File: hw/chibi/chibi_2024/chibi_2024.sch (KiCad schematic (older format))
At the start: 85 parts, among them P1 VIN, P3 GND, P4 CONN_02X05, P5 SWD, Q1 AO3415A, Q10 Q_NPN_CBE, Q11 Q_NPN_CBE, Q2 AO3415A, Q3 AO3415A, Q4 AO3415A, Q5 AO3415A, Q6 AO3415A, Q7 AO3415A, Q8 AO3415A, Q9 Q_PNP_CBE, SW1 USER, SW2 RESET, U1 LD1117S33CTR, U2 SP3485CN, U3 STM32F030F4Px, U4 LM358, U5 74HC595_mine, U6 LM393, U7 74HC595_mine, Y1 8MHz

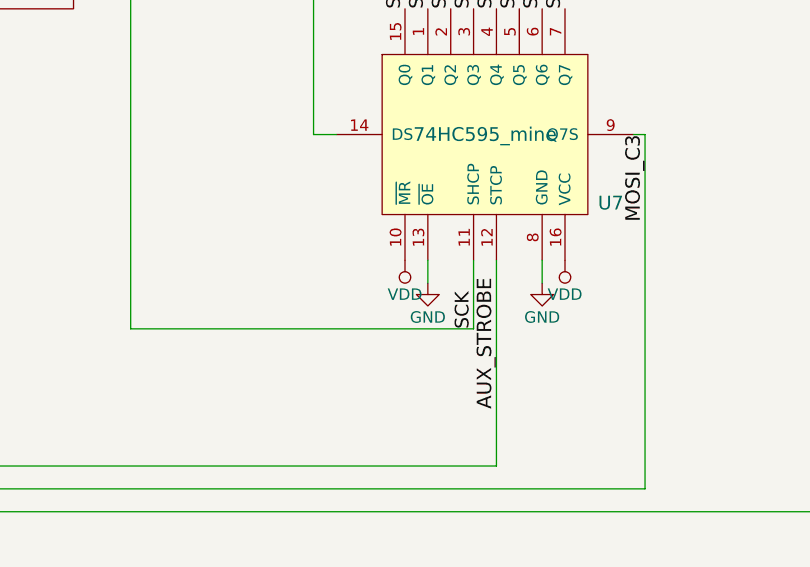
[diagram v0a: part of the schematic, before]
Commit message: Layout mostly done
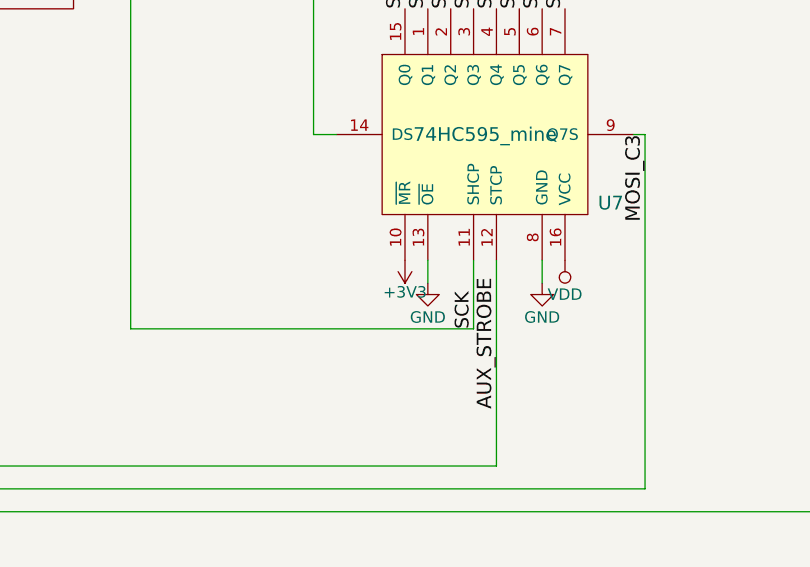
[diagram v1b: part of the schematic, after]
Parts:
- C19, C3: footprint Capacitors_ThroughHole:C_Radial_D10_L20_P5-7.5 -> Capacitors_ThroughHole:C_Radial_D10_L20_P5
- D1: footprint Discret:D5 -> Discret:D3
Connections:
- net +3V3: now also U7.10 (~MR)
- net VDD: no longer U7.10 (~MR)
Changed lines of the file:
@@
 F 0 "C3" H 15200 4150 50  0000 L CNN
 F 1 "1000u" H 15150 3900 50  0000 L CNN
-F 2 "Capacitors_ThroughHole:C_Radial_D10_L20_P5-7.5" H 15438 3850 50  0001 C CNN
+F 2 "Capacitors_ThroughHole:C_Radial_D10_L20_P5" H 15438 3850 50  0001 C CNN
 F 3 "" H 15400 4000 50  0000 C CNN
 F 4 "RAD FR 1.000/25" H 15400 3750 60  0000 C CNN "Reichelt"
@@
 	1    13000 12700
 	-1   0    0    -1
-$EndComp
-$Comp
-L VDD #PWR018
-U 1 1 5903D437
-P 12900 12600
-F 0 "#PWR018" H 12900 12450 50  0001 C CNN
-F 1 "VDD" H 12900 12750 50  0000 C CNN
-F 2 "" H 12900 12600 50  0000 C CNN
-F 3 "" H 12900 12600 50  0000 C CNN
-	1    12900 12600
-	1    0    0    1
 $EndComp
 $Comp
@@
 F 0 "C19" H 14750 10150 50  0000 L CNN
 F 1 "1000u" H 14700 9900 50  0000 L CNN
-F 2 "Capacitors_ThroughHole:C_Radial_D10_L20_P5-7.5" H 14988 9850 50  0001 C CNN
+F 2 "Capacitors_ThroughHole:C_Radial_D10_L20_P5" H 14988 9850 50  0001 C CNN
 F 3 "" H 14950 10000 50  0000 C CNN
 	1    14950 10000
@@
 F 0 "D1" H 14800 4100 50  0000 C CNN
 F 1 "6.4V 1.3W" V 15000 4000 50  0000 C CNN
-F 2 "Discret:D5" H 14800 4000 50  0001 C CNN
+F 2 "Discret:D3" H 14800 4000 50  0001 C CNN
 F 3 "" H 14800 4000 50  0000 C CNN
 	1    14800 4000
@@
 Wire Wire Line
 	5850 12000 4600 12000
+$Comp
+L +3V3 #PWR?
+U 1 1 590A17BD
+P 12900 12600
+F 0 "#PWR?" H 12900 12450 50  0001 C CNN
+F 1 "+3V3" H 12900 12740 50  0000 C CNN
+F 2 "" H 12900 12600 50  0000 C CNN
+F 3 "" H 12900 12600 50  0000 C CNN
+	1    12900 12600
+	-1   0    0    1
+$EndComp
 $EndSCHEMATC

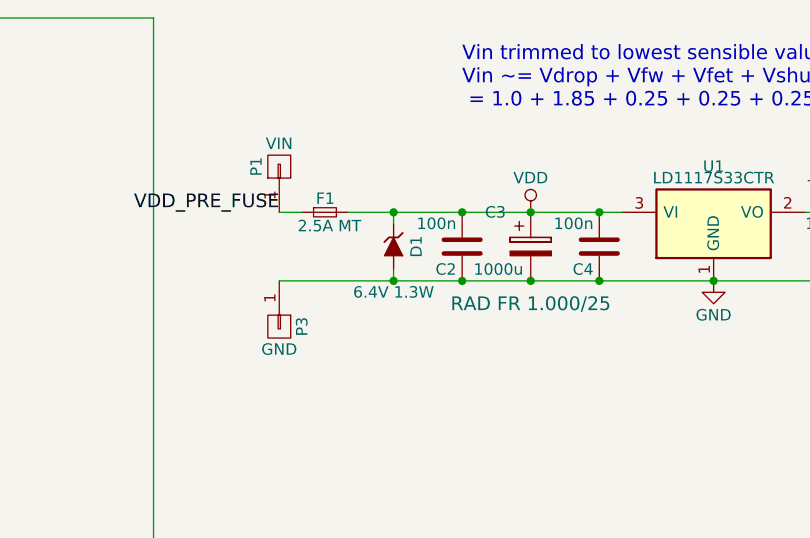
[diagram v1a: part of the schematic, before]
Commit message: Design mostly done
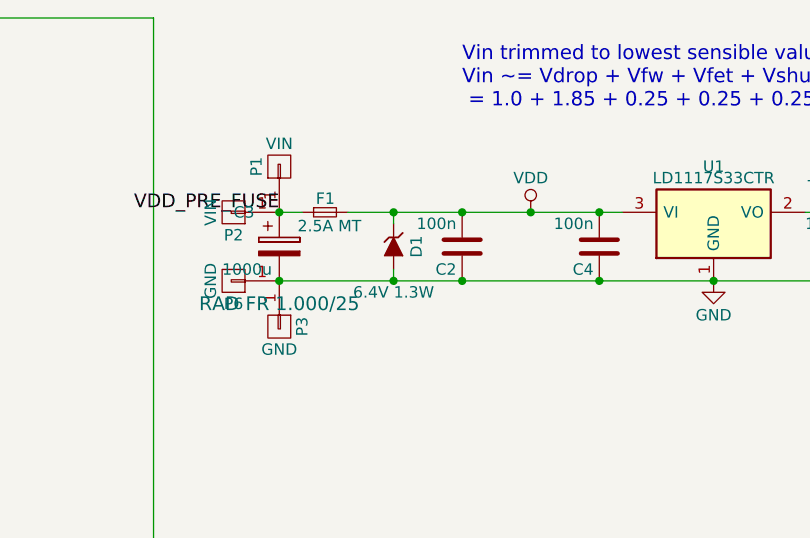
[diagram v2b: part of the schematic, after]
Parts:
- added P2: VIN, footprints:spade_6.35mm, symbol CONN_01X01
- added P6: GND, footprints:spade_6.35mm, symbol CONN_01X01
- SW1, SW2: footprint Buttons_Switches_ThroughHole:SW_PUSH_SMALL -> Buttons_Switches_SMD:SW_SPST_FSMSM
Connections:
- net GND: now also P6.1 (P1)
- net VDD: no longer C3.1
- net VDD_PRE_FUSE: now also C3.1, P2.1 (P1)
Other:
- moved on the sheet: C3
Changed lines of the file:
@@
 L CP C3
 U 1 1 5901F62F
-P 15400 4000
-F 0 "C3" H 15200 4150 50  0000 L CNN
-F 1 "1000u" H 15150 3900 50  0000 L CNN
-F 2 "Capacitors_ThroughHole:C_Radial_D10_L20_P5" H 15438 3850 50  0001 C CNN
-F 3 "" H 15400 4000 50  0000 C CNN
-F 4 "RAD FR 1.000/25" H 15400 3750 60  0000 C CNN "Reichelt"
-	1    15400 4000
+P 14300 4000
+F 0 "C3" H 14100 4150 50  0000 L CNN
+F 1 "1000u" H 14050 3900 50  0000 L CNN
+F 2 "Capacitors_ThroughHole:C_Radial_D10_L20_P5" H 14338 3850 50  0001 C CNN
+F 3 "" H 14300 4000 50  0000 C CNN
+F 4 "RAD FR 1.000/25" H 14300 3750 60  0000 C CNN "Reichelt"
+	1    14300 4000
 	1    0    0    -1
 $EndComp
@@
 $EndComp
 $Comp
-L GND #PWR019
+L GND #PWR018
 U 1 1 5905739D
 P 4850 13300
-F 0 "#PWR019" H 4850 13050 50  0001 C CNN
+F 0 "#PWR018" H 4850 13050 50  0001 C CNN
 F 1 "GND" H 4850 13150 50  0000 C CNN
 F 2 "" H 4850 13300 50  0000 C CNN
@@
 $EndComp
 $Comp
-L +3V3 #PWR020
+L +3V3 #PWR019
 U 1 1 59059547
 P 2750 3850
-F 0 "#PWR020" H 2750 3700 50  0001 C CNN
+F 0 "#PWR019" H 2750 3700 50  0001 C CNN
 F 1 "+3V3" H 2750 3990 50  0000 C CNN
 F 2 "" H 2750 3850 50  0000 C CNN
@@
 $EndComp
 $Comp
-L GND #PWR021
+L GND #PWR020
 U 1 1 5905B96D
 P 7150 6800
-F 0 "#PWR021" H 7150 6550 50  0001 C CNN
+F 0 "#PWR020" H 7150 6550 50  0001 C CNN
 F 1 "GND" H 7150 6650 50  0000 C CNN
 F 2 "" H 7150 6800 50  0000 C CNN
@@
 $EndComp
 $Comp
-L +3V3 #PWR022
+L +3V3 #PWR021
 U 1 1 5905BCF8
 P 7050 6300
-F 0 "#PWR022" H 7050 6150 50  0001 C CNN
+F 0 "#PWR021" H 7050 6150 50  0001 C CNN
 F 1 "+3V3" H 7050 6440 50  0000 C CNN
 F 2 "" H 7050 6300 50  0000 C CNN
@@
 $EndComp
 $Comp
-L VDD #PWR023
+L VDD #PWR022
 U 1 1 5905CD8E
 P 15400 3850
-F 0 "#PWR023" H 15400 3700 50  0001 C CNN
+F 0 "#PWR022" H 15400 3700 50  0001 C CNN
 F 1 "VDD" H 15400 4000 50  0000 C CNN
 F 2 "" H 15400 3850 50  0000 C CNN
@@
 F 0 "SW1" H 7730 3810 50  0000 C CNN
 F 1 "USER" H 7650 3650 50  0000 C CNN
-F 2 "Buttons_Switches_ThroughHole:SW_PUSH_SMALL" H 7650 3900 50  0001 C CNN
+F 2 "Buttons_Switches_SMD:SW_SPST_FSMSM" H 7650 3900 50  0001 C CNN
 F 3 "" H 7650 3900 50  0000 C CNN
 	1    7650 3700
@@
 F 0 "SW2" H 3080 4810 50  0000 C CNN
 F 1 "RESET" H 3000 4650 50  0000 C CNN
-F 2 "Buttons_Switches_ThroughHole:SW_PUSH_SMALL" H 3000 4900 50  0001 C CNN
+F 2 "Buttons_Switches_SMD:SW_SPST_FSMSM" H 3000 4900 50  0001 C CNN
 F 3 "" H 3000 4900 50  0000 C CNN
 	1    3000 4700
@@
 $EndComp
 $Comp
-L GND #PWR024
+L GND #PWR023
 U 1 1 59065530
 P 14950 10250
-F 0 "#PWR024" H 14950 10000 50  0001 C CNN
+F 0 "#PWR023" H 14950 10000 50  0001 C CNN
 F 1 "GND" H 14950 10100 50  0000 C CNN
 F 2 "" H 14950 10250 50  0000 C CNN
@@
 CM_STAGE2_FB
 $Comp
-L VDD #PWR025
+L VDD #PWR024
 U 1 1 5906AB80
 P 16200 6800
-F 0 "#PWR025" H 16200 6650 50  0001 C CNN
+F 0 "#PWR024" H 16200 6650 50  0001 C CNN
 F 1 "VDD" H 16200 6950 50  0000 C CNN
 F 2 "" H 16200 6800 50  0000 C CNN
@@
 $EndComp
 $Comp
-L GND #PWR026
+L GND #PWR025
 U 1 1 5906CB51
 P 15750 6500
-F 0 "#PWR026" H 15750 6250 50  0001 C CNN
+F 0 "#PWR025" H 15750 6250 50  0001 C CNN
 F 1 "GND" H 15750 6350 50  0000 C CNN
 F 2 "" H 15750 6500 50  0000 C CNN
@@
 $EndComp
 $Comp
-L GND #PWR027
+L GND #PWR026
 U 1 1 5906EF8A
 P 16700 6500
-F 0 "#PWR027" H 16700 6250 50  0001 C CNN
+F 0 "#PWR026" H 16700 6250 50  0001 C CNN
 F 1 "GND" H 16700 6350 50  0000 C CNN
 F 2 "" H 16700 6500 50  0000 C CNN
@@
 CMEAS_OFFX_COMP
 $Comp
-L GND #PWR028
+L GND #PWR027
 U 1 1 59071D5D
 P 7750 3950
-F 0 "#PWR028" H 7750 3700 50  0001 C CNN
+F 0 "#PWR027" H 7750 3700 50  0001 C CNN
 F 1 "GND" H 7750 3800 50  0000 C CNN
 F 2 "" H 7750 3950 50  0000 C CNN
@@
 $EndComp
 $Comp
-L +3V3 #PWR029
+L +3V3 #PWR028
 U 1 1 590927CA
 P 16950 7600
-F 0 "#PWR029" H 16950 7450 50  0001 C CNN
+F 0 "#PWR028" H 16950 7450 50  0001 C CNN
 F 1 "+3V3" H 16950 7740 50  0000 C CNN
 F 2 "" H 16950 7600 50  0000 C CNN
@@
 Vin trimmed to lowest sensible value to reduce power dissipation.\nVin ~~= Vdrop + Vfw + Vfet + Vshunt + Vwiring\n = 1.0 + 1.85 + 0.25 + 0.25 + 0.25 = 3.6V
 $Comp
-L +3V3 #PWR030
+L +3V3 #PWR029
 U 1 1 59098A31
 P 8550 5050
-F 0 "#PWR030" H 8550 4900 50  0001 C CNN
+F 0 "#PWR029" H 8550 4900 50  0001 C CNN
 F 1 "+3V3" H 8550 5190 50  0000 C CNN
 F 2 "" H 8550 5050 50  0000 C CNN
@@
 $EndComp
 $Comp
-L +3V3 #PWR031
+L +3V3 #PWR030
 U 1 1 590D225D
 P 6900 9900
-F 0 "#PWR031" H 6900 9750 50  0001 C CNN
+F 0 "#PWR030" H 6900 9750 50  0001 C CNN
 F 1 "+3V3" H 6900 10040 50  0000 C CNN
 F 2 "" H 6900 9900 50  0000 C CNN
@@
 $EndComp
 $Comp
-L GND #PWR032
+L GND #PWR031
 U 1 1 590E4406
 P 7750 13000
-F 0 "#PWR032" H 7750 12750 50  0001 C CNN
+F 0 "#PWR031" H 7750 12750 50  0001 C CNN
 F 1 "GND" H 7750 12850 50  0000 C CNN
 F 2 "" H 7750 13000 50  0000 C CNN
@@
 SCK
 $Comp
-L +3V3 #PWR033
+L +3V3 #PWR032
 U 1 1 590F5DC8
 P 5450 10850
-F 0 "#PWR033" H 5450 10700 50  0001 C CNN
+F 0 "#PWR032" H 5450 10700 50  0001 C CNN
 F 1 "+3V3" V 5350 10900 50  0000 C CNN
 F 2 "" H 5450 10850 50  0000 C CNN
@@
 $EndComp
 $Comp
-L GND #PWR034
+L GND #PWR033
 U 1 1 590F5FC2
 P 5550 10850
-F 0 "#PWR034" H 5550 10600 50  0001 C CNN
+F 0 "#PWR033" H 5550 10600 50  0001 C CNN
 F 1 "GND" H 5550 10700 50  0000 C CNN
 F 2 "" H 5550 10850 50  0000 C CNN
@@
 $EndComp
 $Comp
-L GND #PWR035
+L GND #PWR034
 U 1 1 590F70E3
 P 6050 10850
-F 0 "#PWR035" H 6050 10600 50  0001 C CNN
+F 0 "#PWR034" H 6050 10600 50  0001 C CNN
 F 1 "GND" H 6050 10700 50  0000 C CNN
 F 2 "" H 6050 10850 50  0000 C CNN
@@
 $EndComp
 $Comp
-L +3V3 #PWR036
+L +3V3 #PWR035
 U 1 1 590F8493
 P 6150 10850
-F 0 "#PWR036" H 6150 10700 50  0001 C CNN
+F 0 "#PWR035" H 6150 10700 50  0001 C CNN
 F 1 "+3V3" V 6250 10900 50  0000 C CNN
 F 2 "" H 6150 10850 50  0000 C CNN
@@
 MOSI_C3
 $Comp
-L GND #PWR037
+L GND #PWR036
 U 1 1 590FF5A0
 P 8900 5150
-F 0 "#PWR037" H 8900 4900 50  0001 C CNN
+F 0 "#PWR036" H 8900 4900 50  0001 C CNN
 F 1 "GND" H 8900 5000 50  0000 C CNN
 F 2 "" H 8900 5150 50  0000 C CNN
@@
 Wire Wire Line
 	14300 4150 18150 4150
-Connection ~ 15400 4150
-Connection ~ 15400 3850
 Wire Wire Line
 	16600 3850 18150 3850
@@
 $EndComp
 $Comp
-L +3V3 #PWR038
+L +3V3 #PWR037
 U 1 1 590B5F7D
 P 19300 11150
-F 0 "#PWR038" H 19300 11000 50  0001 C CNN
+F 0 "#PWR037" H 19300 11000 50  0001 C CNN
 F 1 "+3V3" H 19300 11290 50  0000 C CNN
 F 2 "" H 19300 11150 50  0000 C CNN
@@
 $EndComp
 $Comp
-L +3V3 #PWR039
+L +3V3 #PWR038
 U 1 1 590AABFE
 P 18300 10800
-F 0 "#PWR039" H 18300 10650 50  0001 C CNN
+F 0 "#PWR038" H 18300 10650 50  0001 C CNN
 F 1 "+3V3" H 18300 10940 50  0000 C CNN
 F 2 "" H 18300 10800 50  0000 C CNN
@@
 $EndComp
 $Comp
-L GND #PWR040
+L GND #PWR039
 U 1 1 590A8B03
 P 16750 12350
-F 0 "#PWR040" H 16750 12100 50  0001 C CNN
+F 0 "#PWR039" H 16750 12100 50  0001 C CNN
 F 1 "GND" H 16750 12200 50  0000 C CNN
 F 2 "" H 16750 12350 50  0000 C CNN
@@
 $EndComp
 $Comp
-L +3V3 #PWR041
+L +3V3 #PWR040
 U 1 1 5908945C
 P 19300 12650
-F 0 "#PWR041" H 19300 12500 50  0001 C CNN
+F 0 "#PWR040" H 19300 12500 50  0001 C CNN
 F 1 "+3V3" H 19300 12790 50  0000 C CNN
 F 2 "" H 19300 12650 50  0000 C CNN
@@
 $EndComp
 $Comp
-L +3V3 #PWR042
+L +3V3 #PWR041
 U 1 1 59089468
 P 18300 12300
-F 0 "#PWR042" H 18300 12150 50  0001 C CNN
+F 0 "#PWR041" H 18300 12150 50  0001 C CNN
 F 1 "+3V3" H 18300 12440 50  0000 C CNN
 F 2 "" H 18300 12300 50  0000 C CNN
@@
 Connection ~ 20200 12950
 $Comp
-L GND #PWR043
+L GND #PWR042
 U 1 1 5908ADC5
 P 18800 12050
-F 0 "#PWR043" H 18800 11800 50  0001 C CNN
+F 0 "#PWR042" H 18800 11800 50  0001 C CNN
 F 1 "GND" H 18800 11900 50  0000 C CNN
 F 2 "" H 18800 12050 50  0000 C CNN
@@
 	19300 13450 18300 13450
 $Comp
-L GND #PWR044
+L GND #PWR043
 U 1 1 5908B7E7
 P 18800 13500
-F 0 "#PWR044" H 18800 13250 50  0001 C CNN
+F 0 "#PWR043" H 18800 13250 50  0001 C CNN
 F 1 "GND" H 18800 13350 50  0000 C CNN
 F 2 "" H 18800 13500 50  0000 C CNN
@@
 $EndComp
 $Comp
-L +3V3 #PWR045
+L +3V3 #PWR044
 U 1 1 5908C10E
 P 20200 10550
-F 0 "#PWR045" H 20200 10400 50  0001 C CNN
+F 0 "#PWR044" H 20200 10400 50  0001 C CNN
 F 1 "+3V3" H 20200 10690 50  0000 C CNN
 F 2 "" H 20200 10550 50  0000 C CNN
@@
 	5850 12000 4600 12000
 $Comp
-L +3V3 #PWR?
+L +3V3 #PWR045
 U 1 1 590A17BD
 P 12900 12600
-F 0 "#PWR?" H 12900 12450 50  0001 C CNN
+F 0 "#PWR045" H 12900 12450 50  0001 C CNN
 F 1 "+3V3" H 12900 12740 50  0000 C CNN
 F 2 "" H 12900 12600 50  0000 C CNN
@@
 	-1   0    0    1
 $EndComp
+$Comp
+L CONN_01X01 P2
+U 1 1 590B536A
+P 14100 3850
+F 0 "P2" H 14100 3950 50  0000 C CNN
+F 1 "VIN" V 14200 3850 50  0000 C CNN
+F 2 "footprints:spade_6.35mm" H 14100 3850 50  0001 C CNN
+F 3 "" H 14100 3850 50  0000 C CNN
+	1    14100 3850
+	-1   0    0    1
+$EndComp
+$Comp
+L CONN_01X01 P6
+U 1 1 590B56E6
+P 14100 4150
+F 0 "P6" H 14100 4250 50  0000 C CNN
+F 1 "GND" V 14200 4150 50  0000 C CNN
+F 2 "footprints:spade_6.35mm" H 14100 4150 50  0001 C CNN
+F 3 "" H 14100 4150 50  0000 C CNN
+	1    14100 4150
+	-1   0    0    1
+$EndComp
+Connection ~ 14300 3850
+Connection ~ 14300 4150
+Connection ~ 15400 3850
 $EndSCHEMATC

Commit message: Release v0.2
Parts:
- P1, P3: footprint Mounting_Holes:MountingHole_4.3mm_M4_Pad_Via -> footprints:m3_pillar
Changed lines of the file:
@@
 F 0 "P1" H 14300 3750 50  0000 C CNN
 F 1 "VIN" V 14400 3650 50  0000 C CNN
-F 2 "Mounting_Holes:MountingHole_4.3mm_M4_Pad_Via" H 14300 3650 50  0001 C CNN
+F 2 "footprints:m3_pillar" H 14300 3650 50  0001 C CNN
 F 3 "" H 14300 3650 50  0000 C CNN
 	1    14300 3650
@@
 F 0 "P3" H 14300 4450 50  0000 C CNN
 F 1 "GND" V 14400 4350 50  0000 C CNN
-F 2 "Mounting_Holes:MountingHole_4.3mm_M4_Pad_Via" H 14300 4350 50  0001 C CNN
+F 2 "footprints:m3_pillar" H 14300 4350 50  0001 C CNN
 F 3 "" H 14300 4350 50  0000 C CNN
 	1    14300 4350

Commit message: Schematic fixed up so far
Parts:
- removed Q10, Q11: Q_NPN_CBE, TO_SOT_Packages_SMD:SOT-23_Handsoldering, symbol Q_NPN_CBE
- removed Q9: Q_PNP_CBE, TO_SOT_Packages_SMD:SOT-23_Handsoldering, symbol Q_PNP_CBE
- removed R12: 10k, Resistors_SMD:R_0603_HandSoldering, symbol R
- added Q?: AO3415A, TO_SOT_Packages_SMD:SOT-23_Handsoldering, symbol Q_PMOS_GSD
- added Q? (x4): Q_NPN_BEC, symbol Q_NPN_BEC
- added Q? (x3): Q_PNP_BEC, symbol Q_PNP_BEC
- added R?: 7R5, Resistors_SMD:R_0603_HandSoldering, symbol R
- added R? (x5): 100k, Resistors_SMD:R_0603_HandSoldering, symbol R
- added R? (x2): 10k, Resistors_SMD:R_0603_HandSoldering, symbol R
- added R?: 1k, Resistors_SMD:R_0603_HandSoldering, symbol R
- added U?: 74HCT125, symbol 74HCT125
- U1: symbol LD1117S33CTR -> LD1117S33CTR-RESCUE-chibi_2024
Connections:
- net SEG_B_CTRL is gone; now on net SEG_A_CTRL: Q3.1 (G), R32.2, U7.6 (Q6)
- net SEG_C_CTRL is gone; now on net SEG_A_CTRL: Q1.1 (G), U7.3 (Q3)
- net SEG_DP_CTRL is gone; now on net SEG_A_CTRL: Q4.1 (G), U7.2 (Q2)
- net SEG_D_CTRL is gone; now on net SEG_A_CTRL: Q6.1 (G), U7.15 (Q0)
- net SEG_F_CTRL is gone; now on net SEG_E_CTRL: Q5.1 (G), U7.7 (Q7)
- net SEG_G_CTLR is gone; now on net SEG_E_CTRL: Q2.1 (G), U7.4 (Q4)
- net +3V3: now also U1.4 (VO); no longer R20.1, R25.2, U3.1 (BOOT0), U6.8 (V+), U6.8 (V+)
- net CM_STAGE1: now also U6.2 (_)
- net GND: now also R10.2, U3.1 (BOOT0), Q?.2 (E), Q?.2 (E), Q?.2 (E), Q?.2 (E), U?.1 (~OE0), U?.10 (~OE2), U?.13 (~OE3), U?.4 (~OE1), U?.7 (GND); no longer R10.1
- net MOSI_C0: now also U5.14 (DS), U?.9 (I2)
- net MOSI_C2: now also U5.9 (Q7S)
- net SCK: now also U?.11 (Q3), U?.12 (I3)
- net SEG_COM_MEAS: now also R?.1
- net STROBE: now also U?.2 (I0)
- net VDD: now also C3.1, R20.1, R25.2, U6.8 (V+), U6.8 (V+), Q?.2 (E), Q?.2 (E), Q?.2 (S), R?.2, U?.14 (VCC); no longer R13.1
- net VDD_PRE_FUSE: no longer C3.1
- net mux_mod_left/R_SET_0: now also Q?.3 (C)
- net mux_mod_left/R_SET_1: now also Q?.3 (C)
- net ~OE: now also U?.5 (I1)
- net at U4.3 (+): now also R10.1, R?.1, R?.1; no longer R10.2
- net at R19.1: now also Q?.1 (B)
- net at R33.1: now also Q?.1 (B)
- net at R34.1: now also Q?.1 (B)
- net at U5.15 (Q0): now also R?.1
- net MOSI_C3: no longer names the net of U7.9 (Q7S)
- net MOSI_C3: no longer U5.9 (Q7S)
- net WD_COMP renamed WD_COMP1
- net WD_COMP1: no longer U6.2 (_)
- new net: Q?.2 (E), Q?.3 (D), R13.1
- new net: Q?.1 (G), R?.1, R?.1
- new net: Q?.1 (B), Q?.3 (C), R?.2
- new net: Q?.3 (C), R?.1
- new net: Q?.1 (B), R?.2 (x3)
- new net: Q?.3 (C), R?.2 (x2)
- new net MOSI_C0_HV: U?.8 (Q2)
- new net STROBE_HV: U?.3 (Q0)
- new net mux_mod_left/~OE: Q?.3 (C), R?.1
- new net ~OE_HV: R?.2, U?.6 (Q1)
- no-connect marks 3 -> 4
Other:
- moved on the sheet: C1, C10, C11, C12, C13, C14, C15, C16, C17, C18, C19, C2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

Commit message: Second board revision
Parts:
- removed C14, C15: 220n, Capacitors_SMD:C_0603_HandSoldering, symbol C
- removed C16, C17: comp, Capacitors_SMD:C_0603_HandSoldering, symbol C
- removed C18: 100n, Capacitors_SMD:C_0603_HandSoldering, symbol C
- removed P4: CONN_02X05, Pin_Headers:Pin_Header_Straight_2x05, symbol CONN_02X05
- removed Q?: AO3415A, TO_SOT_Packages_SMD:SOT-23_Handsoldering, symbol Q_PMOS_GSD
- removed Q? (x2): Q_NPN_BEC, symbol Q_NPN_BEC
- removed Q? (x2): Q_PNP_BEC, symbol Q_PNP_BEC
- removed R10, R16: 47k, Resistors_SMD:R_0603_HandSoldering, symbol R
- removed R11, R? (x5): 100k, Resistors_SMD:R_0603_HandSoldering, symbol R
- removed R13: 0.1, Resistors_SMD:R_2512_HandSoldering, symbol R
- removed R14, R15, R2, R? (x2): 10k, Resistors_SMD:R_0603_HandSoldering, symbol R
- removed R17, R18, R6, R7, R8: 4k7, Resistors_SMD:R_0603_HandSoldering, symbol R
- removed R9: 1k, Resistors_SMD:R_0603_HandSoldering, symbol R
- removed R?: 7R5, Resistors_SMD:R_0603_HandSoldering, symbol R
- removed SW1: USER, Buttons_Switches_SMD:SW_SPST_FSMSM, symbol SW_PUSH_SMALL_H
- removed U4: LM358, Housings_SOIC:SOIC-8_3.9x4.9mm_Pitch1.27mm, symbol LM358
- removed Y1: 8MHz, Crystals:Crystal_HC49-SD_SMD, symbol Crystal_Small
- added P4: CONN_02X03, Socket_Strips:Socket_Strip_Straight_2x03, symbol CONN_02X03
- added Y1: 25M, footprints:CRYSTAL-SMD-5X3, symbol Crystal_Small_5x3
- Q14, Q15, Q16: renamed from Q?; footprint (none) -> TO_SOT_Packages_SMD:SOT-23_Handsoldering
- R1: value 10k -> 47k
- U10: renamed from U?; footprint (none) -> Housings_SOIC:SOIC-14_3.9x8.7mm_Pitch1.27mm
- gave numbers to parts that had none: 1
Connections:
- net labels added: ~OE_HV_CB
- net labels removed: CMEAS_OFFX_COMP, CMEAS_OUT, CM_STAGE1, CM_STAGE1_FB, CM_STAGE2_FB, SEG_COM_MEAS, USER_BTN
- wire segments 301 -> 218
- no-connect marks 4 -> 2
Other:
- note removed: "2.5A/250mV FS"
- note removed: "Current measurement"
- note removed: "LED voltage measurement"
- note removed: "PD 0.625W FS"
- moved on the sheet: C10, C2, C3, C4, C5, C6, C7, C8, C9, D1, F1, P1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
